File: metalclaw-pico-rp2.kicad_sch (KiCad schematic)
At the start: 117 parts, among them J1 USB_C_Receptacle_USB2.0_14P, J2 Conn_02x05_Odd_Even, SW1 SW_Push, SW2 SW_Push, U1 XC6220B331MR, U2 RP2354B, U3 APS6404L-3SQRx-SN, Y1 XRCGB40M000F1S2FR0

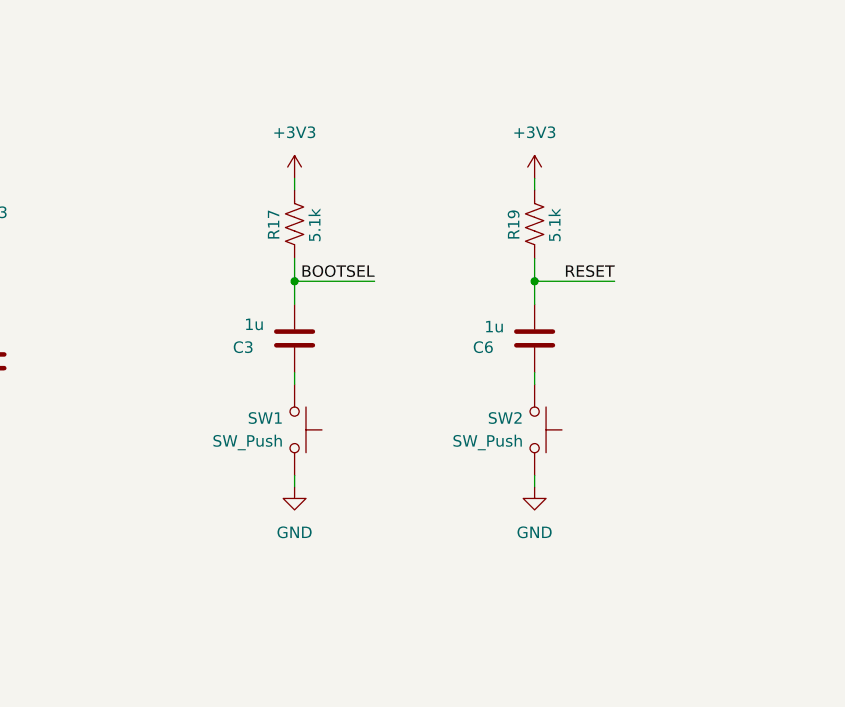
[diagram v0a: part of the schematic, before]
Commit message: Fix reset circuit
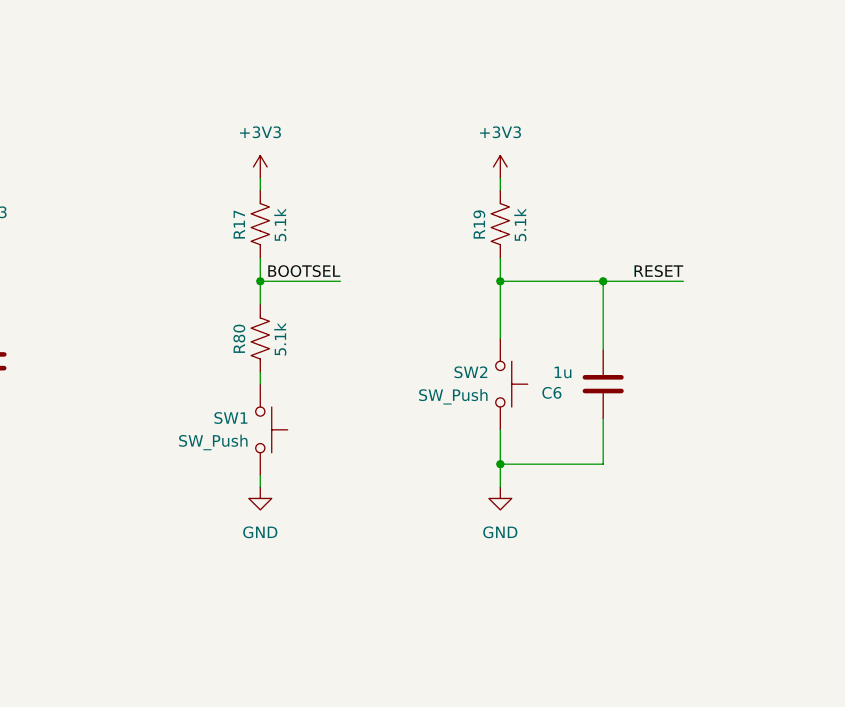
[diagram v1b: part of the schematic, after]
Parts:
- removed C3: 1u, Capacitor_SMD:C_0201_0603Metric, symbol Device:C
- added R80: 5.1k, Resistor_SMD:R_0201_0603Metric, symbol Device:R_US
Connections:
- net BOOTSEL: now also R80.1
- net GND: now also C6.1
- net RESET: now also SW2.2
- net at SW1.2: now also R80.2
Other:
- moved on the sheet: C6, R17, R19, SW1, SW2
